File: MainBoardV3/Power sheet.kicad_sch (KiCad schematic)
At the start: 22 parts, among them J12 Conn_01x02, J13 Conn_01x02, J14 Conn_01x02, J15 Conn_01x02, J16 Conn_01x02, J17 Conn_01x02, J6 Conn_01x02, U1 TSR_2-2450, U3 TSR_2-2433, U4 TEN_50-2411WI

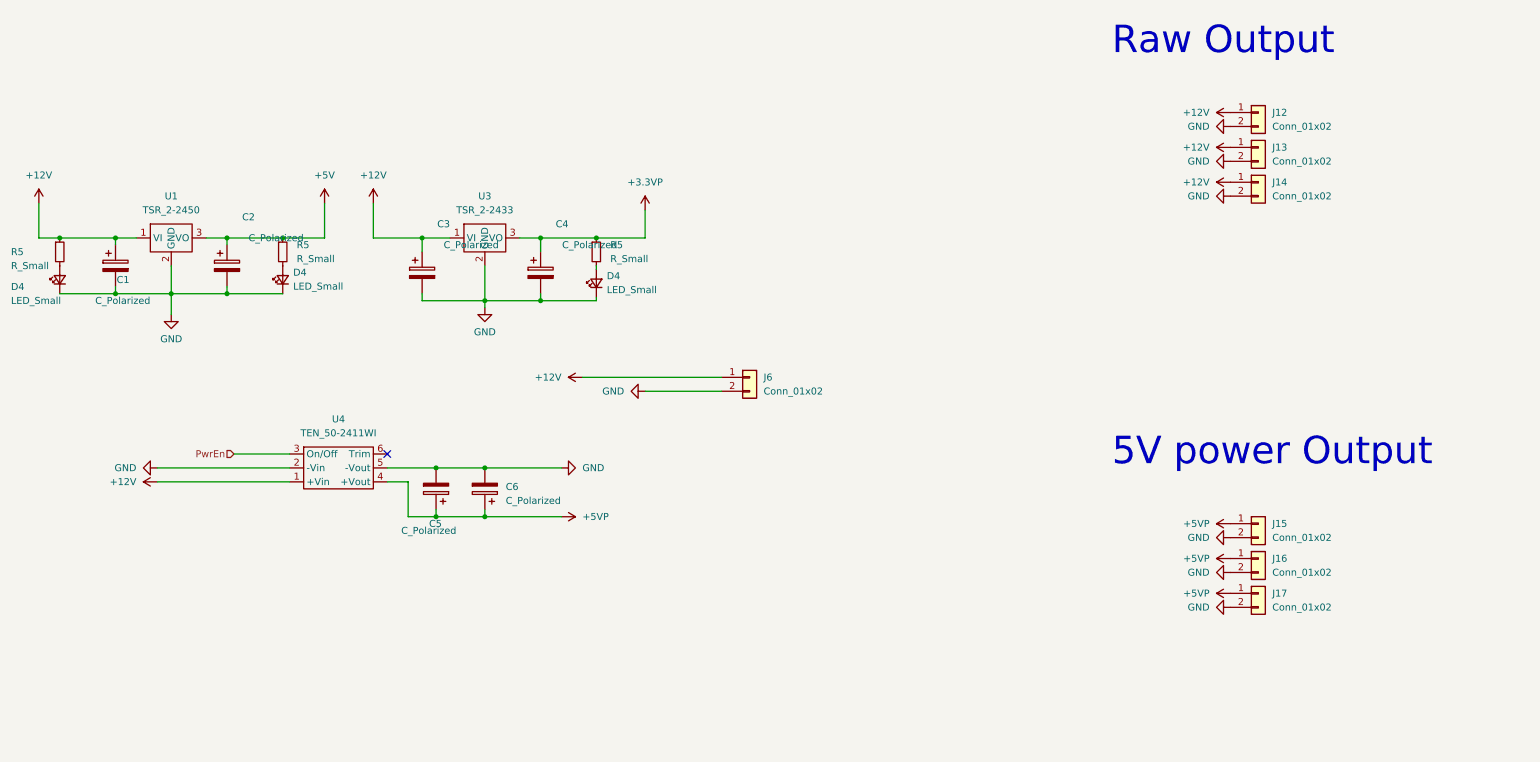
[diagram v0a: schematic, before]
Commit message: Mise a jour pour remi
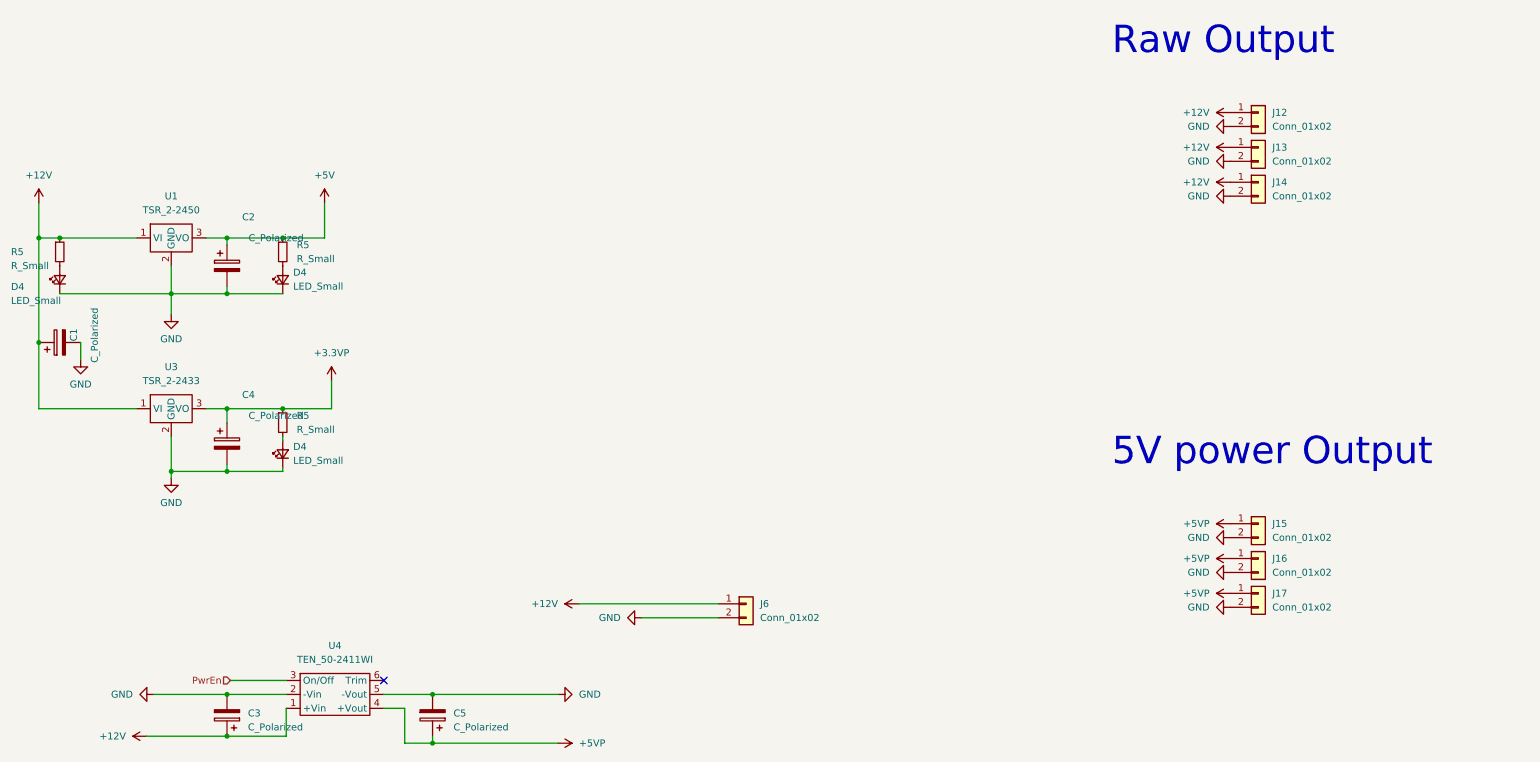
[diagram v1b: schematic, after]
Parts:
- removed C6: C_Polarized, symbol Device:C_Polarized
- C1, C2, C4: footprint (none) -> Capacitor_THT:CP_Radial_D5.0mm_P2.50mm
- C3: footprint (none) -> Capacitor_THT:CP_Radial_D8.0mm_P3.80mm
- C5: footprint (none) -> Capacitor_THT:CP_Radial_D8.0mm_P3.50mm
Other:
- moved on the sheet: C1, C4, C5, D4, J6, R5, U3, U4
